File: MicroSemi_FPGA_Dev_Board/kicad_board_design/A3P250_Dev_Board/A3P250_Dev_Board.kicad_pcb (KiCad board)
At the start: 4 copper layers, 46.7 x 46.7 mm, 50 parts, among them J1 Conn_01x20, J2 Conn_01x20, J3 Conn_01x20, J4 Conn_01x20, U1 A3P250, U2 LTC3561A, U3 LT1962-3.3, X1 ASE-25MHz

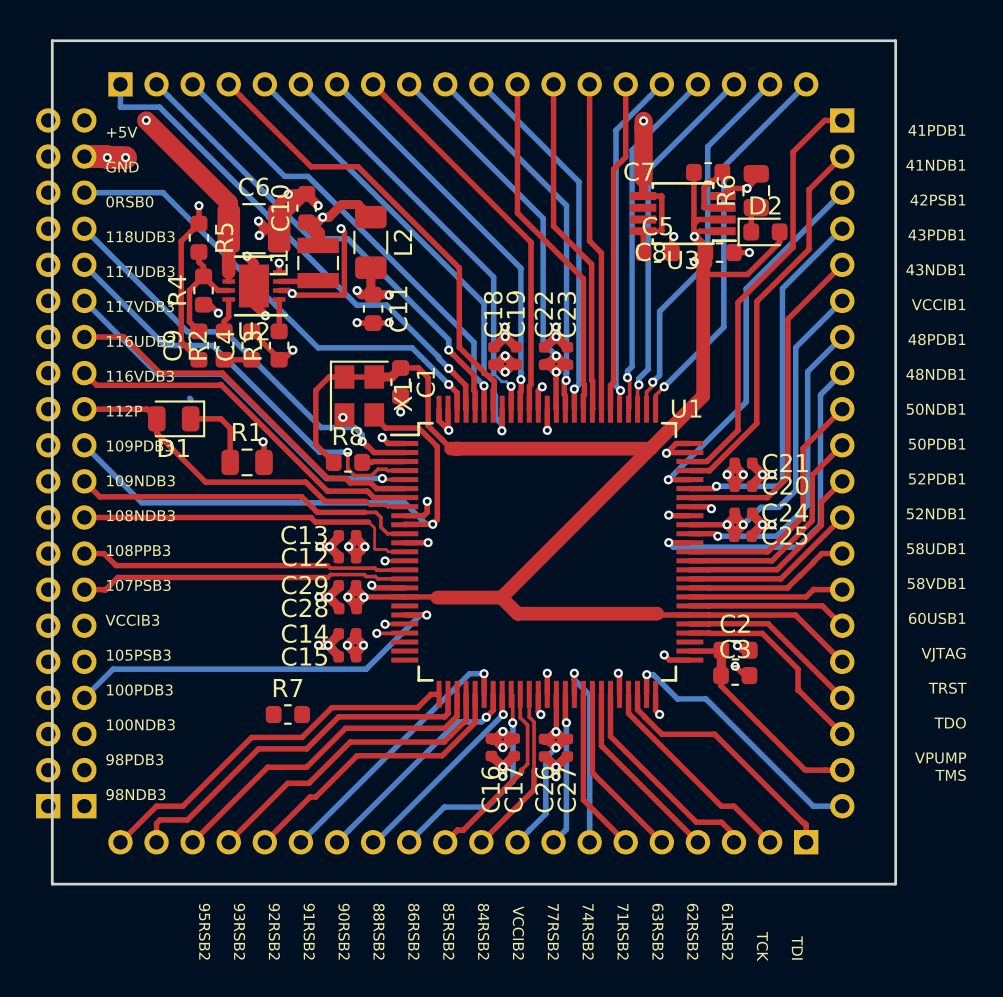
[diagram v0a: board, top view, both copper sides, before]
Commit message: Routed, fixed labels, added test points.
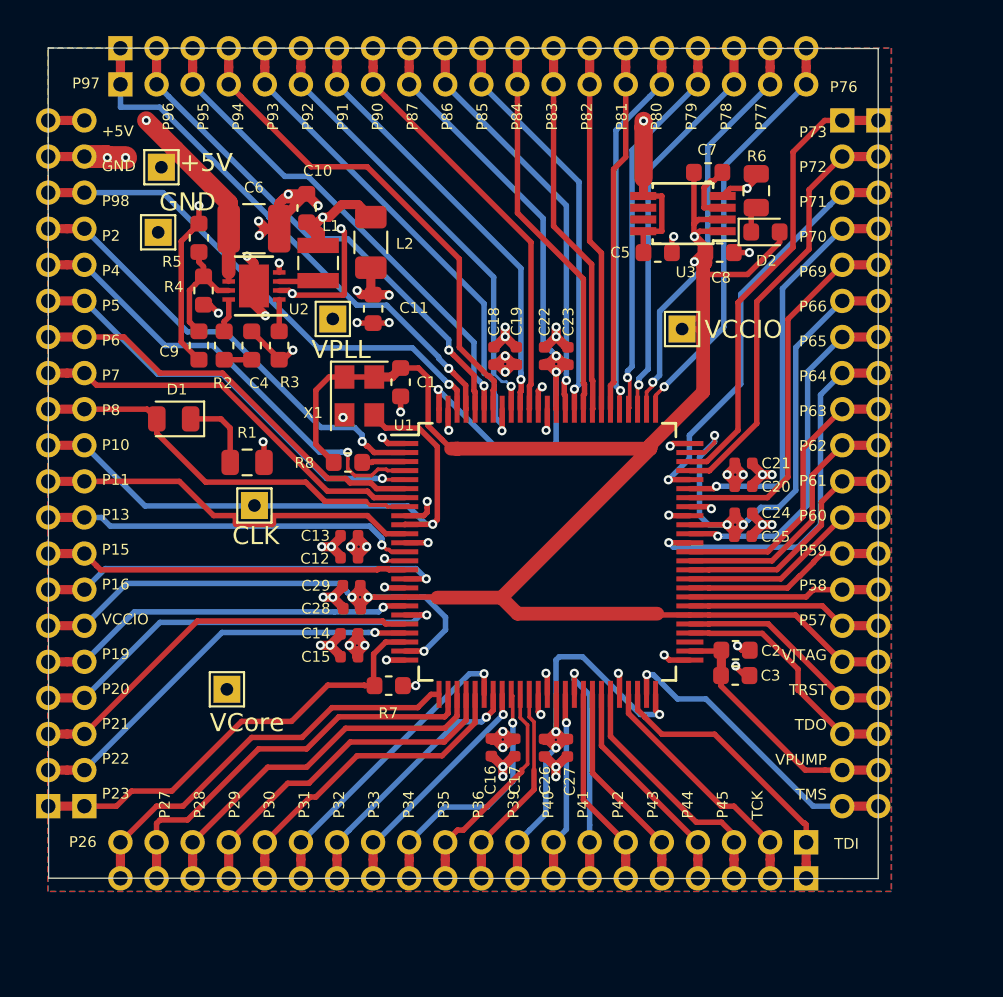
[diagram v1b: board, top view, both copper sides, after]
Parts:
- added +5V: +5V, TestPoint:TestPoint_THTPad_1.5x1.5mm_Drill0.7mm, F.Cu at (107.1, 92.9)
- added CLK: VCCIO, TestPoint:TestPoint_THTPad_1.5x1.5mm_Drill0.7mm, F.Cu at (112.3, 111.6)
- added GND: GND, TestPoint:TestPoint_THTPad_1.5x1.5mm_Drill0.7mm, F.Cu at (107.0, 96.5)
- added J1: Conn_01x20, Connector_PinHeader_2.00mm:PinHeader_1x20_P2.00mm_Vertical, F.Cu at (104.9, 86.3)
- added J2: Conn_01x20, Connector_PinHeader_2.00mm:PinHeader_1x20_P2.00mm_Vertical, F.Cu at (146.9, 90.3)
- added J3: Conn_01x20, Connector_PinHeader_2.00mm:PinHeader_1x20_P2.00mm_Vertical, F.Cu at (142.9, 132.3)
- added VCCIO: VCCIO, TestPoint:TestPoint_THTPad_1.5x1.5mm_Drill0.7mm, F.Cu at (136.0, 101.8)
- added VCore: 1.5V Core, TestPoint:TestPoint_THTPad_1.5x1.5mm_Drill0.7mm, F.Cu at (110.8, 121.8)
- added VPLL: 1.5V PLL, TestPoint:TestPoint_THTPad_1.5x1.5mm_Drill0.7mm, F.Cu at (116.6, 101.3)
- moved R7 5.81 mm to (119.7, 121.6)
- moved J4 2.00 mm to (100.9, 128.3)
- moved J4 2.00 mm to (102.9, 128.3)
- moved C28 0.23 mm to (117.7, 117.3)
- moved C29 0.23 mm to (117.7, 116.1)
- moved C12 0.10 mm to (117.6, 114.5)
- moved C13 0.10 mm to (117.6, 113.3)
- moved C14 0.10 mm to (117.6, 118.7)
- moved C15 0.10 mm to (117.6, 120.0)
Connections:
- U1 pad 100: GND -> Net-(C22-Pad1)
- U1 pad 24: GND -> VCCIB3
- U1 pad 50: GND -> Net-(C26-Pad1)
- U1 pad 74: GND -> Net-(C24-Pad1)
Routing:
- net VCCIB3: track 100.1 -> 129.8 mm, vias 4 -> 5
- net Net-(J4-Pad1): track 0.00 -> 23.6 mm
- net Net-(J4-Pad2): track 1.56 -> 22.2 mm
- net Net-(J4-Pad3): track 1.10 -> 21.7 mm, vias 1 -> 0
- net Net-(J4-Pad5): track 0.00 -> 20.3 mm, vias 0 -> 1
- net Net-(C22-Pad1): track 27.0 -> 42.6 mm, vias 2 -> 3
- net Net-(C26-Pad1): track 14.7 -> 28.9 mm, vias 2 -> 3
- net Net-(C24-Pad1): track 23.9 -> 34.4 mm, vias 2 -> 3
- net Net-(J1-Pad2): track 26.5 -> 30.4 mm
- net Net-(J1-Pad1): track 28.2 -> 32.1 mm
- net Net-(J4-Pad7): track 18.2 -> 22.2 mm, vias 0 -> 1
- net +5V: track 53.4 -> 56.0 mm
- net Net-(J1-Pad4): track 25.7 -> 27.9 mm
- net TMS: track 15.0 -> 17.0 mm
- net VPUMP: track 12.4 -> 14.4 mm
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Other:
- board size 46.7 x 46.7 mm -> 46 x 46 mm
- board text added: "+5V GND P98 P2 P4 P5 P6 P7 P8 P10 P11 P13 P15 P16 VCCIO P19 P20 P21 P22 P23"
- board text added: "P26"
- board text added: "P27 P28 P29 P30 P31 P32 P33 P34 P35 P36 P39 P40 P41 P42 P43 P44 P45 TCK"
- board text added: "P73 P72 P71 P70 P69 P66 P65 P64 P63 P62 P61 P60 P59 P58 P57 VJTAG TRST TDO VPUMP TMS"
- board text added: "P76"
- board text added: "P96 P95 P94 P93 P92 P91 P90 P87 P86 P85 P84 P83 P82 P81 P80 P79 P78 P77"
- board text added: "P97"
- board text added: "TDI"
- board text removed: "+5V GND 0RSB0 118UDB3 117UDB3 117VDB3 116UDB3 116VDB3 112P 109PDB3 109NDB3 108NDB3 108PPB3 107PSB3 VCCIB3 105PSB3 100PDB3 100NDB3 98PDB3 98NDB3"
- board text removed: "41PDB1 41NDB1 42PSB1 43PDB1 43NDB1 VCCIB1 48PDB1 48NDB1 50NDB1 50PDB1 52PDB1 52NDB1 58UDB1 58VDB1 60USB1 VJTAG TRST TDO VPUMP TMS"
- board text removed: "TDI TCK 61RSB2 62RSB2 63RSB2 71RSB2 74RSB2 77RSB2 VCCIB2 84RSB2 85RSB2 86RSB2 88RSB2 90RSB2 91RSB2 92RSB2 93RSB2 95RSB2"
